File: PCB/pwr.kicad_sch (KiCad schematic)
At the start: 21 parts, among them J1 UJ2-MIBH2-4-SMT-TR, J5 Conn_01x02, J6 Conn_01x02, Q1 AO3401A, U2 LTC4412xS6, U3 USBLC6-2P6, U4 TPS62172DSG

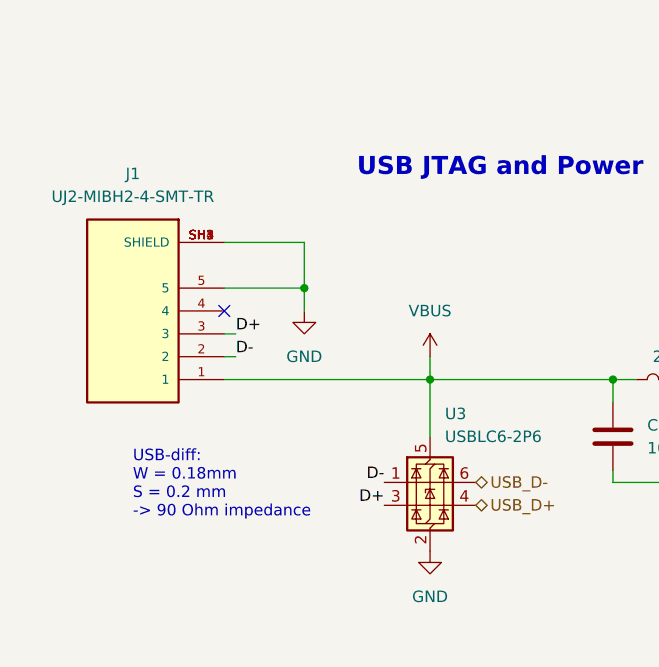
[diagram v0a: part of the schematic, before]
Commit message: Production files
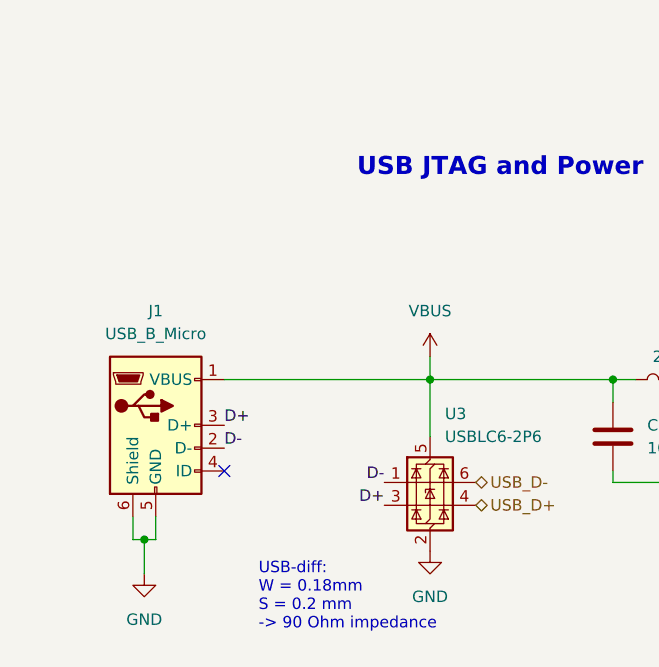
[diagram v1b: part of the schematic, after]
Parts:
- removed J1: UJ2-MIBH2-4-SMT-TR, UJ2-MIBH2-4-SMT-TR:CUI_UJ2-MIBH2-4-SMT-TR, symbol UJ2-MIBH2-4-SMT-TR:UJ2-MIBH2-4-SMT-TR
- added J1: USB_B_Micro, Connector_USB:USB_Micro-B_Molex-105017-0001, symbol Connector:USB_B_Micro
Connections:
- net D+: now also J1.3 (D+)
- net D-: now also J1.2 (D-)
- net GND: now also J1.5 (GND), J1.6 (Shield)
- net VBUS: now also J1.1 (VBUS)
